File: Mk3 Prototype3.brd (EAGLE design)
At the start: 119.6 x 68 mm, 152 parts, among them IC1 TPD3E001DRL, IC2 TPS62082, IC3 STM32F401V, IC4 BQ24092, IC6 CC3100MOD, IC7 BQ2970, IC8 LSM6DS3, IC9 LIS3MDL, J1 ZX62-AB-5PA(11), J2 ER-CON50HT-1, J3 SWD_SHROUD, Q1 DMMT5401, Q2 CSD25402Q3A, Q3 CSD13202Q2, Q4 CSD85301Q2, Q6 CSD25402Q3A, Q8 CSD13202Q2, SW1 JOYSTICK_MINI_MULTICOMP, U1 USD-SOCKET-SDIODM3AT_0011, U2 ER-TFT024-3, X3 ABS07-32.768KHZ-T

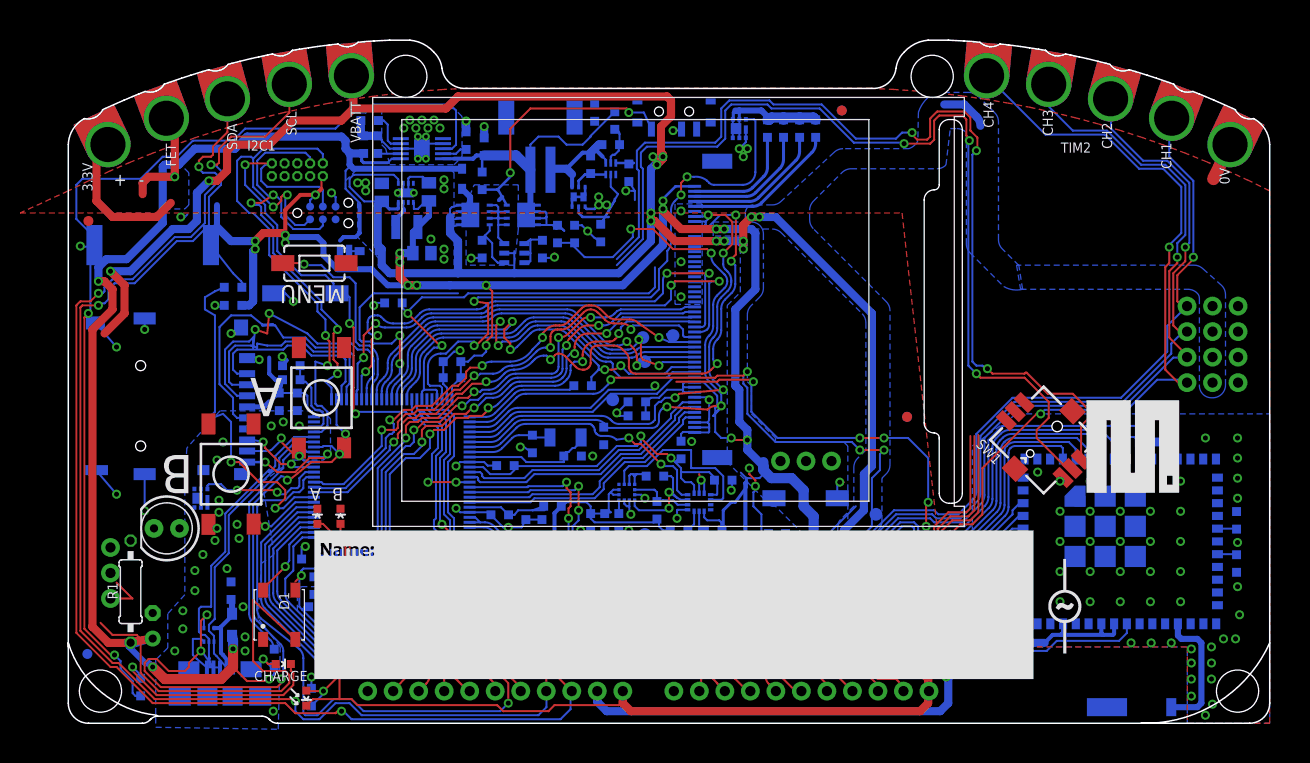
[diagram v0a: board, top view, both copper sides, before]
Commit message: getting there
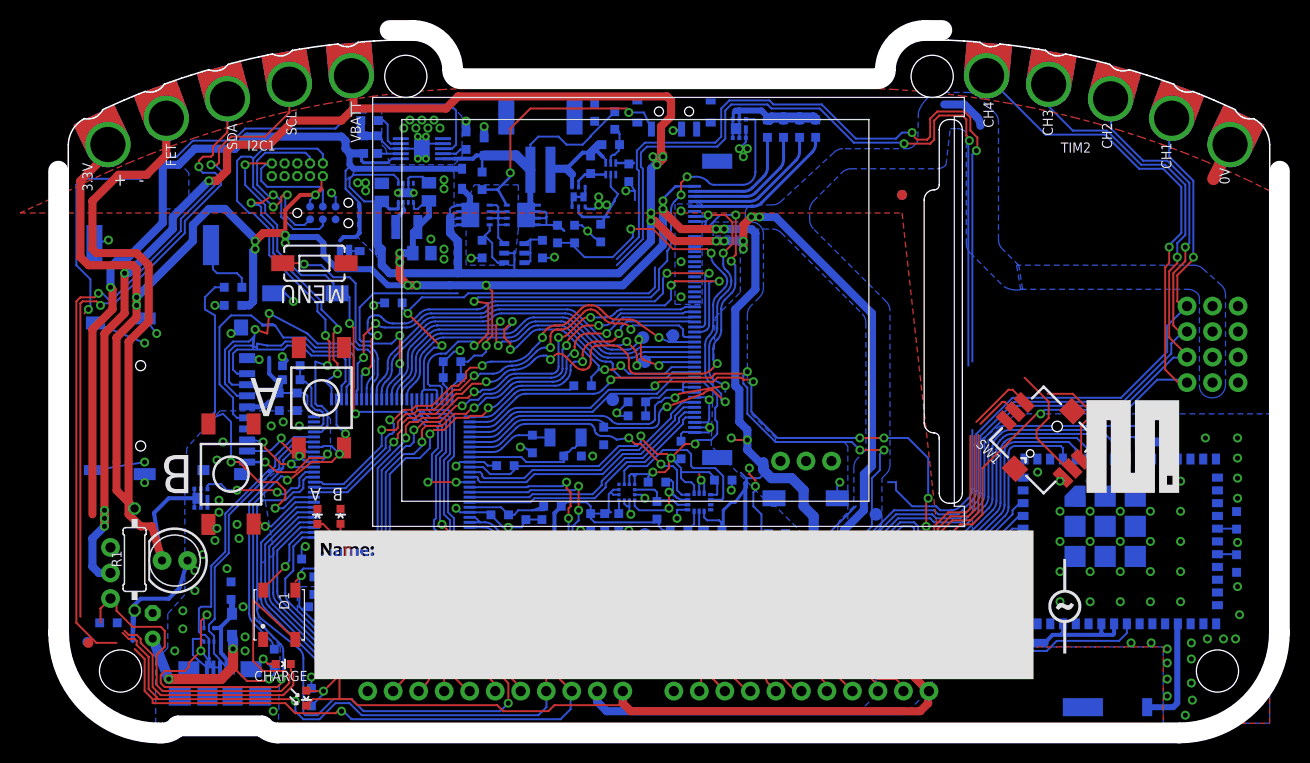
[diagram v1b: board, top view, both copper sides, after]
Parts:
- removed FID2, FID5: FIDUCIAL1X2.5-STOP, TiLDA Mk3 Parts:FIDUCIAL-1X2.5-STOP
- moved FID3 42.0 mm to (2.00, 8.00)
- moved FID1 10.3 mm to (83.0, 52.6)
- moved FID6 10.3 mm to (83.0, 52.6)
- moved R2 7.16 mm to (4.00, 10.0), turned to 0 degrees
- moved LED1 3.30 mm to (10.6, 16.2)
- moved R1 3.22 mm to (6.60, 16.3)
- moved ANT1 2.40 mm to (106.9, 1.60)
- moved FID4 1.20 mm to (1.90, 8.10)
- moved R31 0.63 mm to (58.6, 24.0)
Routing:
- net +3V3: track 505.7 -> 575.4 mm, vias 27 -> 31
- net FET_OUT: track 10.8 -> 70.0 mm, vias 1 -> 0
- net N$9: track 101.4 -> 59.9 mm, vias 2 -> 1
- net VBUS: track 134.3 -> 110.8 mm
- net ADC_VIN: track 40.1 -> 55.2 mm, vias 2 -> 4
- net V_UNREG: track 284.3 -> 299.2 mm, vias 17 -> 20
- net N$60: track 0.00 -> 14.7 mm
- net JOY_RIGHT: track 122.4 -> 113.5 mm, vias 5 -> 4
- net JOY_DOWN: track 103.5 -> 110.2 mm
- net BOOT0: track 137.9 -> 131.8 mm, vias 5 -> 4
- net USART1_RX: track 99.8 -> 105.3 mm
- net USART1_TX: track 96.1 -> 100.7 mm
- net USB_ID: track 63.1 -> 58.9 mm
- net I2C_SCL: track 160.0 -> 155.9 mm
- net TIM2_CH2: track 133.8 -> 137.7 mm
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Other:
- board size 119.6 x 68 mm -> 121.6 x 70 mm
